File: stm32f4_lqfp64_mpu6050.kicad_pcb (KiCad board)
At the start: 4 copper layers, 130 x 100 mm, 82 parts, among them M5 ALIS-CUSTOM-PARTS_POWERPADS, P1 CONN_01X08, P2 CONN_02X08, Q5 BSS138, Q6 CRYSTAL_50X32, U1 STM32F405R, U2 MPU6050, U3 LP2985LV, U4 LP2985LV, U5 W25Q80BV, U6 LM1881, U7 TS5A3160, U8 TS5A3160, X1 CON-JST_SM04B-SRSS-TB, X2 CON-JST_SM04B-SRSS-TB, X3 CON-JST_SM04B-SRSS-TB, X4 CON-JST_SM04B-SRSS-TB

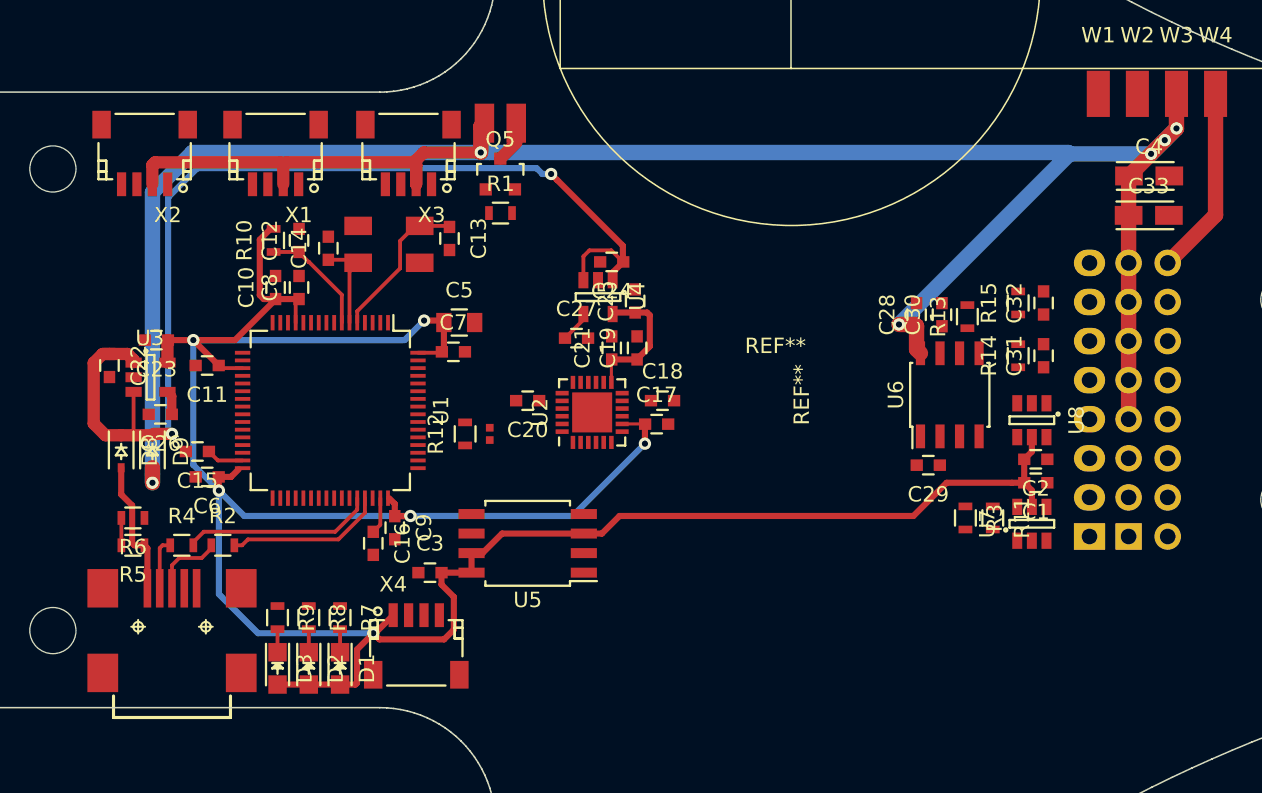
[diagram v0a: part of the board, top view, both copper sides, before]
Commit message: routing done except for ground, but ugly
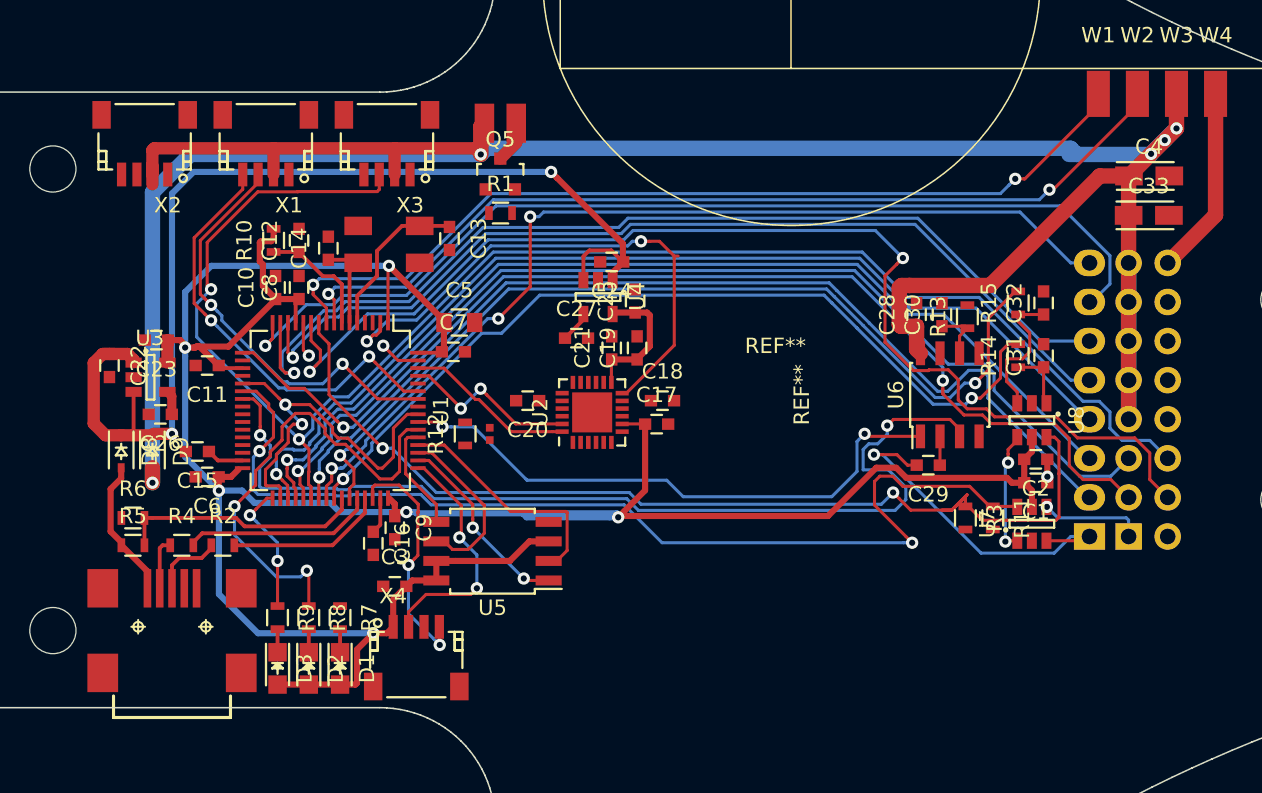
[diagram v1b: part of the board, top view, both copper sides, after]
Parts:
- moved C3 2.45 mm to (119.4, 117.1)
- moved U5 2.34 mm to (125.7, 114.8)
- moved X3 1.53 mm to (118.9, 88.4)
- moved X1 0.90 mm to (111.0, 88.4)
- moved X4 0.76 mm to (120.8, 121.7)
- moved X2 0.64 mm to (103.1, 88.4)
- turned R5 to 0 degrees
- turned R6 to 0 degrees
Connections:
- C26 pad 1: reg_bypass -> Net-(C26-Pad1)
- C27 pad 1: reg_bypass -> Net-(C27-Pad1)
- U3 pad 4: reg_bypass -> Net-(C26-Pad1)
- U4 pad 4: reg_bypass -> Net-(C27-Pad1)
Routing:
- net TIM8_CH2/FRSKY_RSSI/DSM: track 0.00 -> 101.9 mm, vias 0 -> 2
- net ADC3: track 0.00 -> 77.1 mm, vias 0 -> 2
- net TIM5_CH4: track 0.00 -> 71.6 mm, vias 0 -> 2
- net TIM8_CH1: track 0.00 -> 68.6 mm, vias 0 -> 1
- net BW_MASK: track 0.00 -> 67.8 mm, vias 0 -> 2
- net TIM12_CH1/PPM: track 0.00 -> 66.3 mm, vias 0 -> 1
- net TIM12_CH2: track 0.00 -> 66.0 mm, vias 0 -> 1
- net BW_LEVEL: track 0.00 -> 65.7 mm, vias 0 -> 2
- net TIM5_CH2: track 0.00 -> 65.4 mm, vias 0 -> 1
- net TIM5_CH3: track 0.00 -> 65.3 mm, vias 0 -> 1
- net TIM8_CH3: track 0.00 -> 65.1 mm, vias 0 -> 1
- net VSYNC_EXTI: track 0.00 -> 63.7 mm, vias 0 -> 2
- net TIM8_CH4: track 0.00 -> 62.4 mm, vias 0 -> 3
- net TIM5_CH1: track 0.00 -> 62.2 mm, vias 0 -> 1
- net ADC1: track 0.00 -> 60.4 mm, vias 0 -> 2
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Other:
- net class Default: clearance 0.25 -> 0.2; trace_width 0.25 -> 0.2
- rule trace_clearance: 0.25 -> 0.2
